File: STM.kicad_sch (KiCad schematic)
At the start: 11 parts, among them J2 CONN HEADER SMD 10POS 1.27MM, U1 STM32C542CCU6

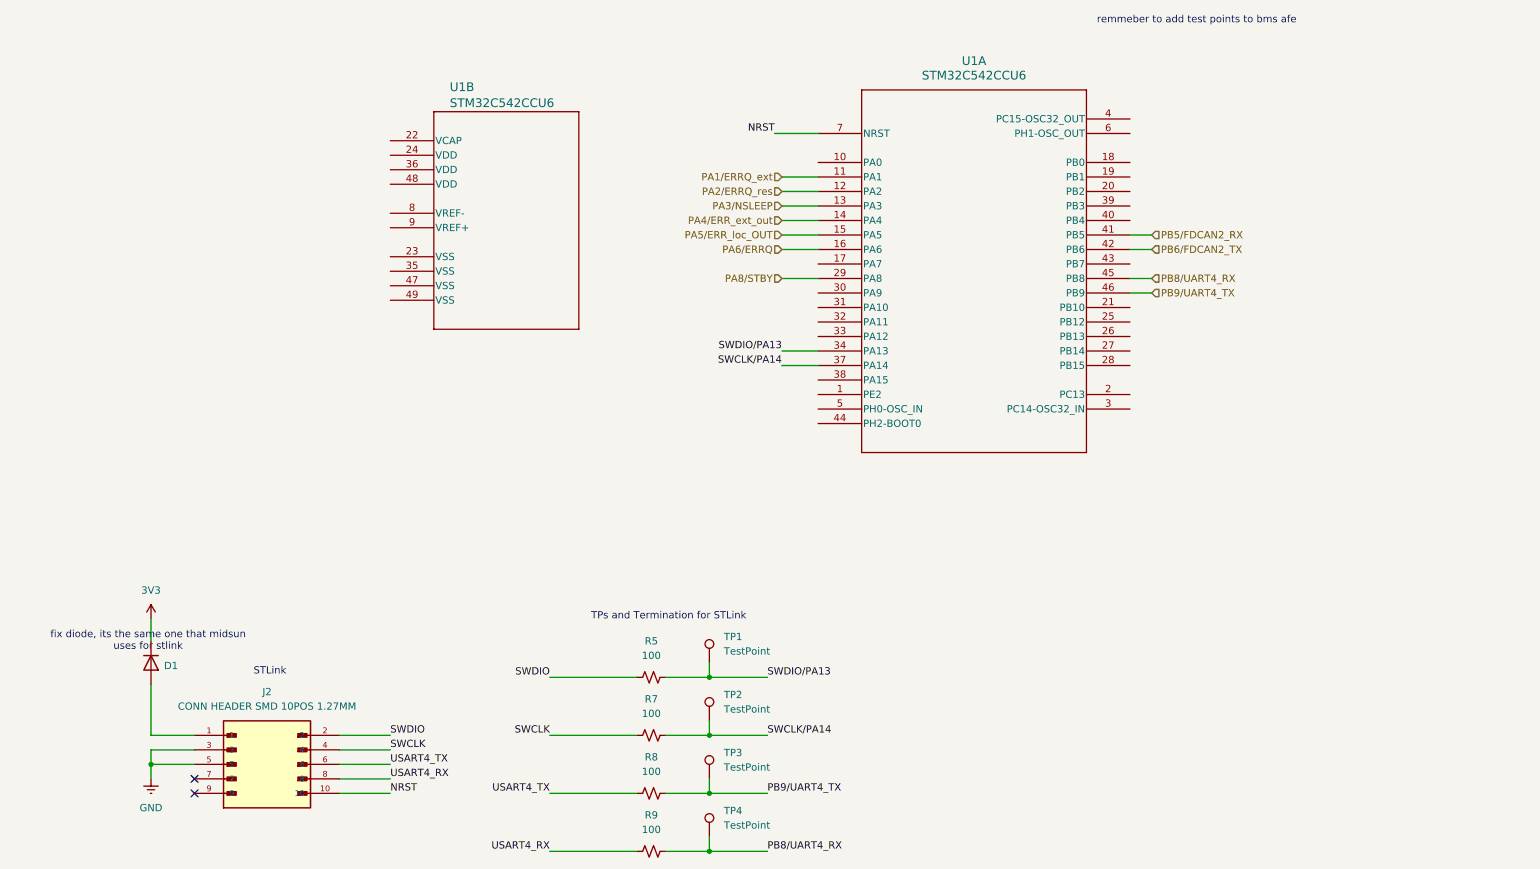
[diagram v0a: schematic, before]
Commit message: schematic done
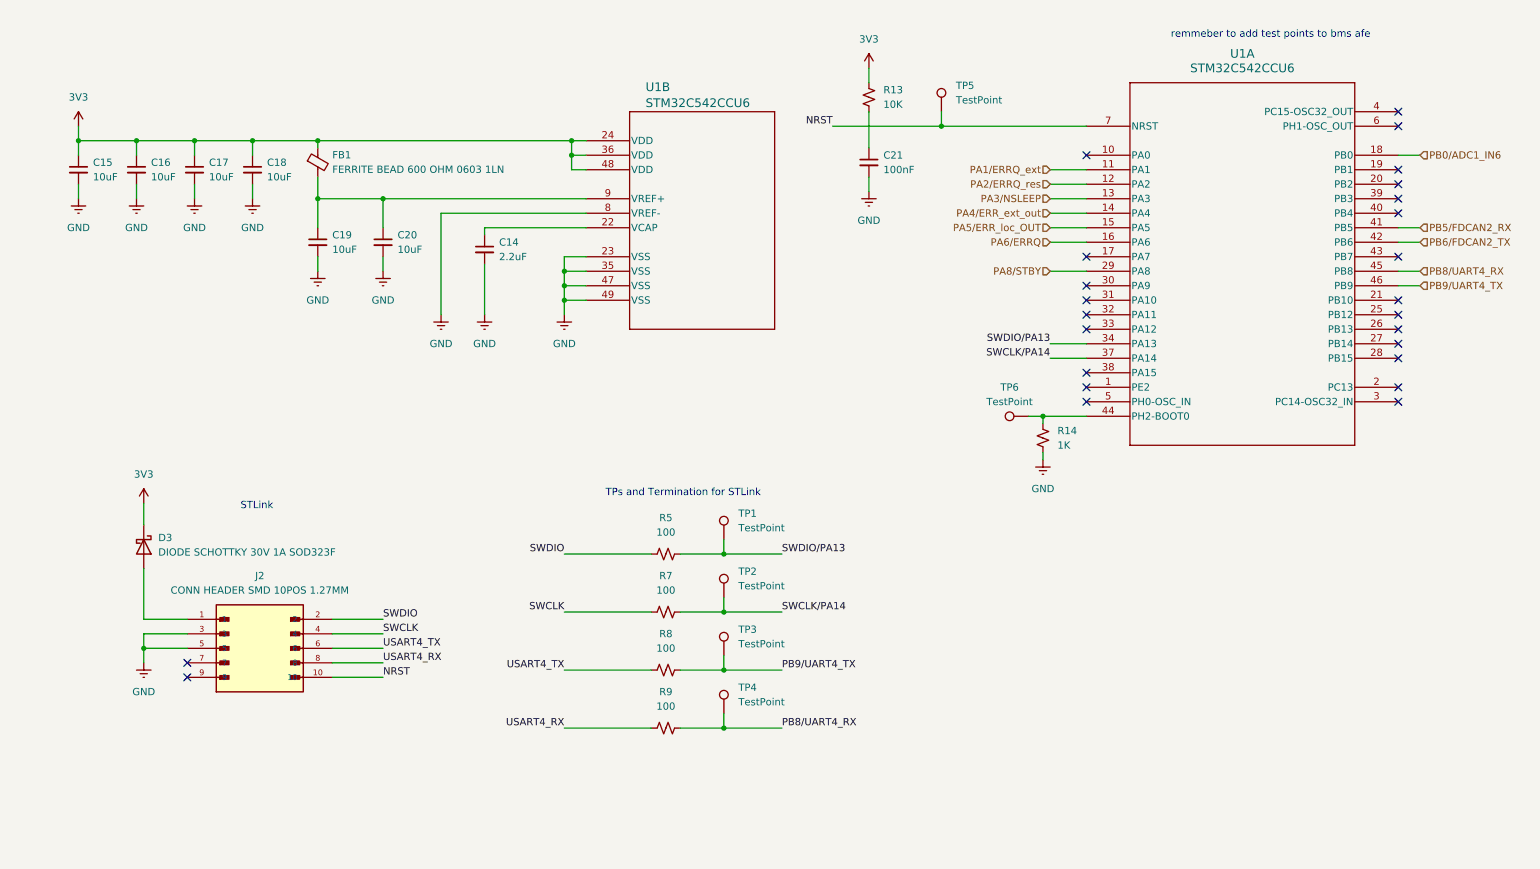
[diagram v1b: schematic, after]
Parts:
- removed D1: (no value), symbol Diode:1N914
- added C14: 2.2uF, symbol Device:C_Small
- added C15, C16, C17, C18, C19, C20: 10uF, symbol Device:C_Small
- added C21: 100nF, symbol Device:C_Small
- added D3: DIODE SCHOTTKY 30V 1A SOD323F, footprints:P39_SOD-323P, symbol symbols:SDB13HS-AQ
- added FB1: FERRITE BEAD 600 OHM 0603 1LN, Resistor_SMD:R_0603_1608Metric, symbol Device:FerriteBead_Small
- added R13: 10K, symbol Device:R_Small_US
- added R14: 1K, symbol Device:R_Small_US
- added TP5, TP6: TestPoint, symbol Connector:TestPoint
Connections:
- net 3V3: now also U1.24 (VDD), U1.36 (VDD), U1.48 (VDD), C15.1, C16.1, C17.1, C18.1, D3.1 (K), FB1.1, R13.1
- net GND: now also U1.23 (VSS), U1.35 (VSS), U1.47 (VSS), U1.49 (VSS), U1.8 (VREF-), C14.2, C15.2, C16.2, C17.2, C18.2, C19.2, C20.2, C21.2, R14.2
- net NRST: now also TP5.1
- net PB0/ADC1_IN6: now reaches U1.18 (PB0)
- net at U1.44 (PH2-BOOT0): now also R14.1, TP6.1
- net at J2.1: now also D3.2 (A)
- net at U1.22 (VCAP): now also C14.1
- net at U1.9 (VREF+): now also C19.1, C20.1, FB1.2
- new net: C21.1, R13.2
- no-connect marks 2 -> 25
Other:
- note removed: "fix diode, its the same one that midsun uses for stlink"
- moved on the sheet: J2, R5, R7, R8, R9, TP1, TP2, TP3, TP4, U1A, U1B
